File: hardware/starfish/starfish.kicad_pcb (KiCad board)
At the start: 4 copper layers, 80 x 70 mm, 164 parts, among them J1 INS, J10 Stemma QT, J2 8P8C_LED_Shielded, J3 CAM, J4 CAMLED, J5 OUT1, J6 BLTOUCH, J7 MOTOR, J8 MOTOR, J9 MOTOR, SW1 BOOTSEL, U1 VX7805-500, U10 TMC2209, U2 MIC5317-3.3, U3 RP2040, U4 W25Q128JVS, U5 74HC2G34, U6 TVS, U7 74HC2G34, U8 TMC2209, U9 TMC2209, Y1 12MHz

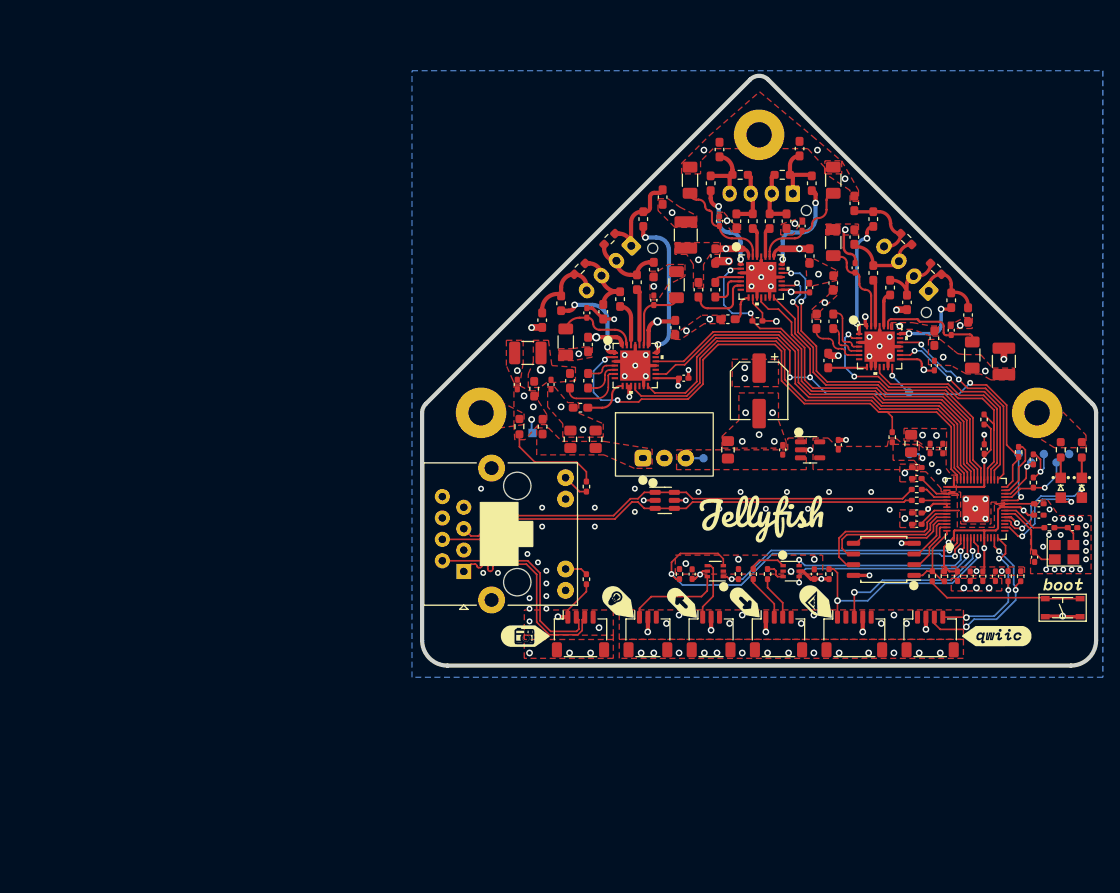
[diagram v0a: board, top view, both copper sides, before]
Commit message: First pass at layout and routing
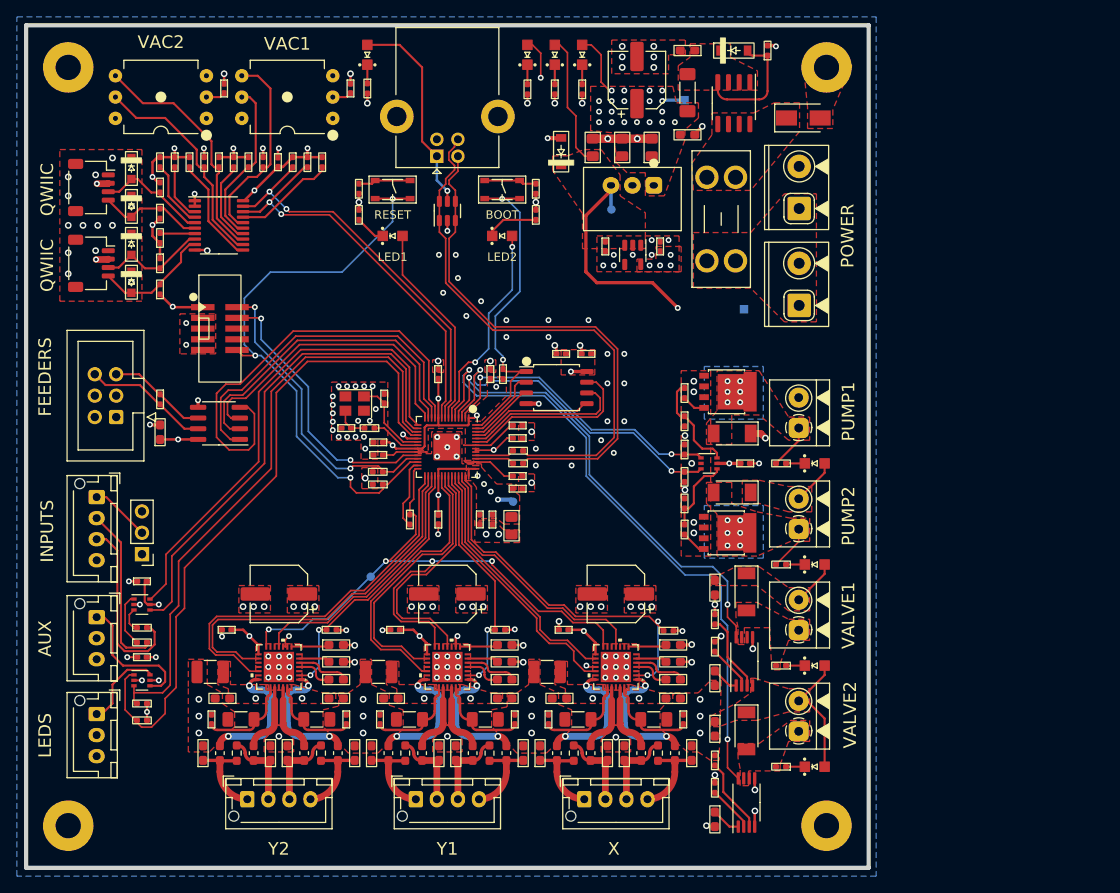
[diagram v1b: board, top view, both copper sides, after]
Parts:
- removed ? (x13): , Graphics
- removed C1, C27, C29, C32, C33, C43, C46, C47, C57, C60, C61, C8, C9: 100n, Capacitor_SMD:C_0402_1005Metric_Pad0.74x0.62mm_HandSolder
- removed C2: 4.7u, Capacitor_SMD:C_0805_2012Metric_Pad1.18x1.45mm_HandSolder
- removed C28, C42, C56: 22n, Capacitor_SMD:C_0603_1608Metric_Pad1.08x0.95mm_HandSolder
- removed C3, C4: 22u, Capacitor_SMD:C_0805_2012Metric_Pad1.18x1.45mm_HandSolder
- removed C30, C36, C37, C44, C50, C51, C58, C64, C65: 100n, Capacitor_SMD:C_0603_1608Metric_Pad1.08x0.95mm_HandSolder
- removed C31, C45, C59: 4.7u, Capacitor_SMD:C_0603_1608Metric_Pad1.08x0.95mm_HandSolder
- removed C35, C49, C63: 10u, Capacitor_SMD:C_1210_3225Metric_Pad1.33x2.70mm_HandSolder
- removed C38, C39, C40, C41, C52, C53, C54, C55, C66, C67, C68, C69: 470p, Capacitor_SMD:C_0603_1608Metric_Pad1.08x0.95mm_HandSolder
- removed C5: 100u, Capacitor_SMD:CP_Elec_6.3x7.7
- removed C6, C7: 1u, Capacitor_SMD:C_0402_1005Metric_Pad0.74x0.62mm_HandSolder
- removed FB1, FB10, FB11, FB12, FB13, FB14, FB2, FB3, FB4, FB5, FB6, FB7, FB8, FB9: 50Ω @ 100MHz, Inductor_SMD:L_0603_1608Metric_Pad1.05x0.95mm_HandSolder
- removed H1, H2, H3: GND, MountingHole:MountingHole_3mm_Pad
- removed J10: Stemma QT, Connector_JST:JST_SH_SM04B-SRSS-TB_1x04-1MP_P1.00mm_Horizontal
- removed J2: 8P8C_LED_Shielded, winterbloom:RJ45_Amphenol_RJE45-188-1411_Vertical
- removed J3: CAM, Connector_JST:JST_SH_SM04B-SRSS-TB_1x04-1MP_P1.00mm_Horizontal
- removed J4: CAMLED, Connector_JST:JST_SH_SM03B-SRSS-TB_1x03-1MP_P1.00mm_Horizontal
- removed J5: OUT1, Connector_JST:JST_SH_SM03B-SRSS-TB_1x03-1MP_P1.00mm_Horizontal
- removed J6: BLTOUCH, Connector_JST:JST_SH_SM05B-SRSS-TB_1x05-1MP_P1.00mm_Horizontal
- removed J7, J8, J9: MOTOR, Connector_JST:JST_XH_B4B-XH-AM_1x04_P2.50mm_Vertical
- removed R1, R15, R2, R26, R27: 5.1k, Resistor_SMD:R_0402_1005Metric_Pad0.72x0.64mm_HandSolder
- removed R13, R14, R20, R23: 10k, Resistor_SMD:R_0402_1005Metric_Pad0.72x0.64mm_HandSolder
- removed R16, R3: 100, Resistor_SMD:R_0402_1005Metric_Pad0.72x0.64mm_HandSolder
- removed R18, R19, R21, R22, R24, R25: 220m, Resistor_SMD:R_1206_3216Metric_Pad1.30x1.75mm_HandSolder
- removed RV1, RV2, RV3, RV4, RV5, RV6, RV7: 35V, Resistor_SMD:R_0603_1608Metric_Pad0.98x0.95mm_HandSolder
- removed TP1: GND, TestPoint:TestPoint_Pad_1.0x1.0mm
- removed TP2: 24V, TestPoint:TestPoint_Pad_1.0x1.0mm
- removed TP3: 5V, TestPoint:TestPoint_Pad_D1.0mm
- removed TP5: GND, TestPoint:TestPoint_Pad_D1.0mm
- removed TP6: 3V3, TestPoint:TestPoint_Pad_D1.0mm
- removed TP7: ~{RST}, TestPoint:TestPoint_Pad_D1.0mm
- removed TP8: SWD, TestPoint:TestPoint_Pad_D1.0mm
- removed TP9: SWC, TestPoint:TestPoint_Pad_D1.0mm
- removed U1: VX7805-500, winterbloom:Converter_DCDC_CUI_VX78-500_THT
- removed U10, U8, U9: TMC2209, winterbloom:TMC2209-LA
- removed U2: MIC5317-3.3, Package_TO_SOT_SMD:SOT-23-5
- removed U5, U7: 74HC2G34, Package_TO_SOT_SMD:SOT-363_SC-70-6
- removed U6: TVS, Package_TO_SOT_SMD:SOT-23-6
- added C1201: 4u7, winterbloom:C_0603_HandSolder, F.Cu at (100.0, 112.1)
- added C1202: 100n, winterbloom:C_0603_HandSolder, F.Cu at (100.0, 101.4)
- added C1301: 4u7, winterbloom:C_0603_HandSolder, F.Cu at (100.0, 128.9)
- added C1302: 100n, winterbloom:C_0603_HandSolder, F.Cu at (100.0, 118.1)
- added C1401: 22n, winterbloom:C_0603_HandSolder, F.Cu at (95.0, 112.3)
- added C1402: 100n, winterbloom:C_0402_HandSolder, F.Cu at (82.0, 106.4)
- added C1403: 100n, winterbloom:C_0603_HandSolder, F.Cu at (95.0, 110.2)
- added C1404: 4u7, winterbloom:C_0603_HandSolder, F.Cu at (95.0, 108.2)
- added C1405: 100n, winterbloom:C_0402_HandSolder, F.Cu at (96.2, 117.0)
- added C1406: 100n, winterbloom:C_0402_HandSolder, F.Cu at (80.2, 117.0)
- added C1407: 470p, winterbloom:C_0603_HandSolder, F.Cu at (89.2, 121.0)
- added C1408: 470p, winterbloom:C_0603_HandSolder, F.Cu at (79.2, 121.0)
- added C1409: 470p, winterbloom:C_0603_HandSolder, F.Cu at (97.2, 121.0)
- added C1410: 470p, winterbloom:C_0603_HandSolder, F.Cu at (87.2, 121.0)
- added C1411: 100u, Capacitor_SMD:CP_Elec_6.3x9.9, F.Cu at (68.2, 102.1)
- added C1412: 10u, winterbloom:C_1210_HandSolder, F.Cu at (80.0, 111.4)
- added C1413: 100n, winterbloom:C_0603_HandSolder, F.Cu at (95.0, 114.5)
- added C1414: 100n, winterbloom:C_0603_HandSolder, F.Cu at (81.5, 114.5)
- added C1501: 22n, winterbloom:C_0603_HandSolder, F.Cu at (75.0, 112.3)
- added C1502: 100n, winterbloom:C_0402_HandSolder, F.Cu at (62.0, 106.4)
- added C1503: 100n, winterbloom:C_0603_HandSolder, F.Cu at (75.0, 110.2)
- added C1504: 4u7, winterbloom:C_0603_HandSolder, F.Cu at (75.0, 108.2)
- added C1505: 100n, winterbloom:C_0402_HandSolder, F.Cu at (76.2, 117.0)
- added C1506: 100n, winterbloom:C_0402_HandSolder, F.Cu at (60.2, 117.0)
- added C1507: 470p, winterbloom:C_0603_HandSolder, F.Cu at (69.2, 121.0)
- added C1508: 470p, winterbloom:C_0603_HandSolder, F.Cu at (59.2, 121.0)
- added C1509: 470p, winterbloom:C_0603_HandSolder, F.Cu at (77.2, 121.0)
- added C1510: 470p, winterbloom:C_0603_HandSolder, F.Cu at (67.2, 121.0)
- added C1511: 100u, Capacitor_SMD:CP_Elec_6.3x9.9, F.Cu at (88.2, 102.1)
- added C1512: 10u, winterbloom:C_1210_HandSolder, F.Cu at (60.0, 111.4)
- added C1513: 100n, winterbloom:C_0603_HandSolder, F.Cu at (75.0, 114.5)
- added C1514: 100n, winterbloom:C_0603_HandSolder, F.Cu at (61.5, 114.5)
- added C1601: 22n, winterbloom:C_0603_HandSolder, F.Cu at (55.0, 112.3)
- added C1602: 100n, winterbloom:C_0402_HandSolder, F.Cu at (42.0, 106.4)
- added C1603: 100n, winterbloom:C_0603_HandSolder, F.Cu at (55.0, 110.2)
- added C1604: 4u7, winterbloom:C_0603_HandSolder, F.Cu at (55.0, 108.2)
- added C1605: 100n, winterbloom:C_0402_HandSolder, F.Cu at (56.2, 117.0)
- added C1606: 100n, winterbloom:C_0402_HandSolder, F.Cu at (40.2, 117.0)
- added C1607: 470p, winterbloom:C_0603_HandSolder, F.Cu at (49.2, 121.0)
- added C1608: 470p, winterbloom:C_0603_HandSolder, F.Cu at (39.2, 121.0)
- added C1609: 470p, winterbloom:C_0603_HandSolder, F.Cu at (57.2, 121.0)
- added C1610: 470p, winterbloom:C_0603_HandSolder, F.Cu at (47.2, 121.0)
- added C1611: 100u, Capacitor_SMD:CP_Elec_6.3x9.9, F.Cu at (48.2, 102.1)
- added C1612: 10u, winterbloom:C_1210_HandSolder, F.Cu at (40.0, 111.4)
- added C1613: 100n, winterbloom:C_0603_HandSolder, F.Cu at (55.0, 114.5)
- added C1614: 100n, winterbloom:C_0603_HandSolder, F.Cu at (41.5, 114.5)
- added C201: 100n, winterbloom:C_0603_HandSolder, F.Cu at (96.7, 37.6)
- added C202: 100n, winterbloom:C_0603_HandSolder, F.Cu at (96.7, 47.6)
- added C203: 100u, Capacitor_SMD:CP_Elec_6.3x9.9, F.Cu at (90.7, 41.1)
- added C206: 4u7, winterbloom:C_0805_HandSolder, F.Cu at (92.5, 49.1)
- added C207: 22u, winterbloom:C_0805_HandSolder, F.Cu at (89.0, 49.1)
- added C208: 22u, winterbloom:C_0805_HandSolder, F.Cu at (85.5, 49.1)
- added C209: 1u, winterbloom:C_0402_HandSolder, F.Cu at (87.0, 60.9)
- added C210: 1u, winterbloom:C_0402_HandSolder, F.Cu at (93.5, 60.9)
- added C401: 100n, winterbloom:C_0402_HandSolder, F.Cu at (31.9, 109.6)
- added C402: 100n, winterbloom:C_0402_HandSolder, F.Cu at (31.9, 100.6)
- added C501: 100n, winterbloom:C_0402_HandSolder, F.Cu at (48.1, 50.9)
- added C601: 100n, winterbloom:C_0402_HandSolder, F.Cu at (56.7, 42.1)
- added C701: 100n, winterbloom:C_0402_HandSolder, F.Cu at (41.7, 42.1)
- added C801: 100n, winterbloom:C_0603_HandSolder, F.Cu at (34.1, 82.9)
- added C901: 100n, winterbloom:C_0402_HandSolder, F.Cu at (103.6, 86.6)
- added D1001: On, winterbloom:LED_0805_Kingbright_APT2012, F.Cu at (111.8, 86.6)
- added D1002: PMEG3030EP, Diode_SMD:D_SOD-128, F.Cu at (102.0, 83.1)
- added D1101: On, winterbloom:LED_0805_Kingbright_APT2012, F.Cu at (111.8, 98.6)
- added D1102: PMEG3030EP, Diode_SMD:D_SOD-128, F.Cu at (102.0, 90.1)
- added D1201: On, winterbloom:LED_0805_Kingbright_APT2012, F.Cu at (111.8, 110.6)
- added D1202: PMEG3030EP, Diode_SMD:D_SOD-128, F.Cu at (103.7, 101.9)
- added D1301: On, winterbloom:LED_0805_Kingbright_APT2012, F.Cu at (111.8, 122.6)
- added D1302: PMEG3030EP, Diode_SMD:D_SOD-128, F.Cu at (103.7, 118.4)
- added D201: SMAJ28A, Diode_SMD:D_SMA, F.Cu at (110.5, 45.6)
- added D202: PDZ16BGWJ, winterbloom:D_SOD-123, F.Cu at (102.2, 37.6)
- added D203: 24V, winterbloom:LED_0805_Kingbright_APT2012, F.Cu at (84.2, 38.1)
- added D204: 5V, winterbloom:LED_0805_Kingbright_APT2012, F.Cu at (81.0, 38.1)
- added D205: 3V3, winterbloom:LED_0805_Kingbright_APT2012, F.Cu at (77.7, 38.1)
- added D401: PESD5V, winterbloom:D_SOD-323, F.Cu at (30.7, 51.6)
- added D402: PESD5V, winterbloom:D_SOD-323, F.Cu at (30.7, 60.6)
- added D403: PESD5V, winterbloom:D_SOD-323, F.Cu at (30.7, 56.1)
- added D404: PESD5V, winterbloom:D_SOD-323, F.Cu at (30.7, 65.1)
- added D405: PMEG2005EGWJ, winterbloom:D_SOD-123, F.Cu at (81.7, 49.6)
- added D406: USB, winterbloom:LED_0805_Kingbright_APT2012, F.Cu at (58.7, 38.1)
- added F201: Fuse, Fuse:Fuseholder_Blade_Mini_Keystone_3568, F.Cu at (99.0, 62.6)
- added FB1401: 120R @ 100MHz, Inductor_SMD:L_0603_1608Metric_Pad1.05x0.95mm_HandSolder, F.Cu at (95.2, 121.0)
- added FB1402: 120R @ 100MHz, Inductor_SMD:L_0603_1608Metric_Pad1.05x0.95mm_HandSolder, F.Cu at (91.2, 121.0)
- added FB1403: 120R @ 100MHz, Inductor_SMD:L_0603_1608Metric_Pad1.05x0.95mm_HandSolder, F.Cu at (85.2, 121.0)
- added FB1404: 120R @ 100MHz, Inductor_SMD:L_0603_1608Metric_Pad1.05x0.95mm_HandSolder, F.Cu at (81.2, 121.0)
- added FB1501: 120R @ 100MHz, Inductor_SMD:L_0603_1608Metric_Pad1.05x0.95mm_HandSolder, F.Cu at (75.2, 121.0)
- added FB1502: 120R @ 100MHz, Inductor_SMD:L_0603_1608Metric_Pad1.05x0.95mm_HandSolder, F.Cu at (71.2, 121.0)
- added FB1503: 120R @ 100MHz, Inductor_SMD:L_0603_1608Metric_Pad1.05x0.95mm_HandSolder, F.Cu at (65.2, 121.0)
- added FB1504: 120R @ 100MHz, Inductor_SMD:L_0603_1608Metric_Pad1.05x0.95mm_HandSolder, F.Cu at (61.2, 121.0)
- added FB1601: 120R @ 100MHz, Inductor_SMD:L_0603_1608Metric_Pad1.05x0.95mm_HandSolder, F.Cu at (55.2, 121.0)
- added FB1602: 120R @ 100MHz, Inductor_SMD:L_0603_1608Metric_Pad1.05x0.95mm_HandSolder, F.Cu at (51.2, 121.0)
- added FB1603: 120R @ 100MHz, Inductor_SMD:L_0603_1608Metric_Pad1.05x0.95mm_HandSolder, F.Cu at (45.2, 121.0)
- added FB1604: 120R @ 100MHz, Inductor_SMD:L_0603_1608Metric_Pad1.05x0.95mm_HandSolder, F.Cu at (41.2, 121.0)
- added FB201: 60R @ 100MHz, Inductor_SMD:L_1806_4516Metric_Pad1.45x1.90mm_HandSolder, F.Cu at (96.7, 42.6)
- added H101: GND, MountingHole:MountingHole_3mm_Pad, F.Cu at (23.2, 39.6)
- added H102: GND, MountingHole:MountingHole_3mm_Pad, F.Cu at (113.2, 39.6)
- added H103: GND, MountingHole:MountingHole_3mm_Pad, F.Cu at (23.2, 129.6)
- added H104: GND, MountingHole:MountingHole_3mm_Pad, F.Cu at (113.2, 129.6)
- added J1001: Pump, winterbloom:TerminalBlock_4UCON_1x02_P3.50mm_Horizontal, F.Cu at (109.9, 82.4)
- added J1101: Pump, winterbloom:TerminalBlock_4UCON_1x02_P3.50mm_Horizontal, F.Cu at (109.9, 94.4)
- added J1201: Valve, winterbloom:TerminalBlock_4UCON_1x02_P3.50mm_Horizontal, F.Cu at (109.9, 106.4)
- added J1301: Valve, winterbloom:TerminalBlock_4UCON_1x02_P3.50mm_Horizontal, F.Cu at (109.9, 118.4)
- added J1401: Motor, Connector_JST:JST_XH_B4B-XH-AM_1x04_P2.50mm_Vertical, F.Cu at (84.5, 126.5)
- added J1501: Motor, Connector_JST:JST_XH_B4B-XH-AM_1x04_P2.50mm_Vertical, F.Cu at (64.5, 126.5)
- added J1601: Motor, Connector_JST:JST_XH_B4B-XH-AM_1x04_P2.50mm_Vertical, F.Cu at (44.5, 126.5)
- added J201: DC in, winterbloom:TerminalBlock_CUI_TB002-500_1x02_P5.00mm_Vertical, F.Cu at (110.0, 56.4)
- added J202: DC thru, winterbloom:TerminalBlock_CUI_TB002-500_1x02_P5.00mm_Vertical, F.Cu at (110.0, 67.9)
- added J401: Cam LED, Connector_JST:JST_XH_B3B-XH-AM_1x03_P2.50mm_Vertical, F.Cu at (26.6, 116.4)
- added J402: Aux out, Connector_JST:JST_XH_B3B-XH-AM_1x03_P2.50mm_Vertical, F.Cu at (26.6, 104.9)
- added J403: Voltage, Connector_PinHeader_2.54mm:PinHeader_1x03_P2.54mm_Vertical, F.Cu at (31.9, 97.4)
- added J404: Inputs, Connector_JST:JST_XH_B4B-XH-AM_1x04_P2.50mm_Vertical, F.Cu at (26.6, 90.6)
- added J405: Qwiic, Connector_JST:JST_SH_SM04B-SRSS-TB_1x04-1MP_P1.00mm_Horizontal, F.Cu at (25.9, 53.9)
- added J406: Qwiic, Connector_JST:JST_SH_SM04B-SRSS-TB_1x04-1MP_P1.00mm_Horizontal, F.Cu at (25.9, 62.9)
- added J407: USB B, winterbloom:USB_B_Receptacle_Horizontal, F.Cu at (67.0, 50.1)
- added J801: Feeders, Connector_IDC:IDC-Header_2x03_P2.54mm_Vertical, F.Cu at (28.9, 81.1)
- added Q1001: PSMN011-30YLC, Package_TO_SOT_SMD:LFPAK56, F.Cu at (101.5, 78.1)
- added Q1101: PSMN011-30YLC, Package_TO_SOT_SMD:LFPAK56, F.Cu at (101.5, 94.9)
- added Q201: DMP3037LSS-13, Package_SO:SOIC-8_3.9x4.9mm_P1.27mm, F.Cu at (102.2, 43.9)
- added R1001: 100k, winterbloom:R_0402_HandSolder, F.Cu at (96.3, 81.6)
- added R1002: 1k, winterbloom:R_0402_HandSolder, F.Cu at (96.3, 78.3)
- added R1003: 5k1, winterbloom:R_0402_HandSolder, F.Cu at (107.8, 86.6)
- added R1101: 100k, winterbloom:R_0402_HandSolder, F.Cu at (96.3, 91.4)
- added R1102: 1k, winterbloom:R_0402_HandSolder, F.Cu at (96.3, 94.5)
- added R1103: 5k1, winterbloom:R_0402_HandSolder, F.Cu at (107.8, 98.6)
- added R1201: 0R, winterbloom:R_0402_HandSolder, F.Cu at (100.0, 105.1)
- added R1202: 47k, winterbloom:R_0402_HandSolder, F.Cu at (100.0, 108.4)
- added R1203: 5k1, winterbloom:R_0402_HandSolder, F.Cu at (107.8, 110.6)
- added R1301: 0R, winterbloom:R_0402_HandSolder, F.Cu at (100.0, 121.9)
- added R1302: 47k, winterbloom:R_0402_HandSolder, F.Cu at (100.0, 125.1)
- added R1303: 5k1, winterbloom:R_0402_HandSolder, F.Cu at (107.8, 122.6)
- added R1402: 120m, Resistor_SMD:R_1206_3216Metric_Pad1.30x1.75mm_HandSolder, F.Cu at (92.7, 117.0)
- added R1403: 120m, Resistor_SMD:R_1206_3216Metric_Pad1.30x1.75mm_HandSolder, F.Cu at (83.7, 117.0)
- added R1501: 10k, winterbloom:R_0402_HandSolder, F.Cu at (74.5, 106.4)
- added R1502: 120m, Resistor_SMD:R_1206_3216Metric_Pad1.30x1.75mm_HandSolder, F.Cu at (72.7, 117.0)
- added R1503: 120m, Resistor_SMD:R_1206_3216Metric_Pad1.30x1.75mm_HandSolder, F.Cu at (63.7, 117.0)
- added R1601: 10k, winterbloom:R_0402_HandSolder, F.Cu at (54.5, 106.4)
- added R1602: 120m, Resistor_SMD:R_1206_3216Metric_Pad1.30x1.75mm_HandSolder, F.Cu at (52.7, 117.0)
- added R1603: 120m, Resistor_SMD:R_1206_3216Metric_Pad1.30x1.75mm_HandSolder, F.Cu at (43.7, 117.0)
- added R201: 47k, winterbloom:R_0402_HandSolder, F.Cu at (106.2, 37.6)
- added R202: 5k1, winterbloom:R_0402_HandSolder, F.Cu at (84.2, 42.2)
- added R203: 1k, winterbloom:R_0402_HandSolder, F.Cu at (81.0, 42.2)
- added R204: 1k, winterbloom:R_0402_HandSolder, F.Cu at (77.7, 42.2)
- added R306: 1k, winterbloom:R_0402_HandSolder, F.Cu at (57.7, 54.0)
- added R401: 10k, winterbloom:R_0402_HandSolder, F.Cu at (31.9, 117.1)
- added R402: 10k, winterbloom:R_0402_HandSolder, F.Cu at (31.9, 115.1)
- added R403: 120R, winterbloom:R_0402_HandSolder, F.Cu at (31.9, 107.9)
- added R404: 120R, winterbloom:R_0402_HandSolder, F.Cu at (31.9, 106.1)
- added R405: 1k, winterbloom:R_0402_HandSolder, F.Cu at (58.7, 42.1)
- added R501: 4k7, winterbloom:R_0402_HandSolder, F.Cu at (51.6, 50.9)
- added R502: 4k7, winterbloom:R_0402_HandSolder, F.Cu at (49.8, 50.9)
- added R503: 10k, winterbloom:R_0402_HandSolder, F.Cu at (53.3, 50.9)
- added R504: 10k, winterbloom:R_0402_HandSolder, F.Cu at (35.8, 50.9)
- added R505: 10k, winterbloom:R_0402_HandSolder, F.Cu at (34.1, 50.9)
- added R506: 4k7, winterbloom:R_0402_HandSolder, F.Cu at (34.1, 53.9)
- added R507: 4k7, winterbloom:R_0402_HandSolder, F.Cu at (34.1, 57.0)
- added R508: 10k, winterbloom:R_0402_HandSolder, F.Cu at (34.1, 59.9)
- added R509: 4k7, winterbloom:R_0402_HandSolder, F.Cu at (34.1, 62.9)
- added R510: 4k7, winterbloom:R_0402_HandSolder, F.Cu at (34.1, 66.0)
- added R511: 10k, winterbloom:R_0402_HandSolder, F.Cu at (37.6, 50.9)
- added R512: 4k7, winterbloom:R_0402_HandSolder, F.Cu at (39.3, 50.9)
- added R513: 4k7, winterbloom:R_0402_HandSolder, F.Cu at (41.1, 50.9)
- added R514: 10k, winterbloom:R_0402_HandSolder, F.Cu at (42.8, 50.9)
- added R515: 4k7, winterbloom:R_0402_HandSolder, F.Cu at (44.6, 50.9)
- added R516: 4k7, winterbloom:R_0402_HandSolder, F.Cu at (46.3, 50.9)
- added R801: 120R, winterbloom:R_0402_HandSolder, F.Cu at (34.1, 79.0)
- added R901: 10k, winterbloom:R_0402_HandSolder, F.Cu at (96.3, 85.0)
- added R902: 10k, winterbloom:R_0402_HandSolder, F.Cu at (96.3, 88.2)
- added RV1401: MOV, Resistor_SMD:R_0603_1608Metric_Pad0.98x0.95mm_HandSolder, F.Cu at (93.2, 121.0)
- added RV1402: MOV, Resistor_SMD:R_0603_1608Metric_Pad0.98x0.95mm_HandSolder, F.Cu at (83.2, 121.0)
- added RV1501: MOV, Resistor_SMD:R_0603_1608Metric_Pad0.98x0.95mm_HandSolder, F.Cu at (73.2, 121.0)
- added RV1502: MOV, Resistor_SMD:R_0603_1608Metric_Pad0.98x0.95mm_HandSolder, F.Cu at (63.2, 121.0)
- added RV1601: MOV, Resistor_SMD:R_0603_1608Metric_Pad0.98x0.95mm_HandSolder, F.Cu at (53.2, 121.0)
- added RV1602: MOV, Resistor_SMD:R_0603_1608Metric_Pad0.98x0.95mm_HandSolder, F.Cu at (43.2, 121.0)
- added SW301: RESET, winterbloom:Tactile_Switch_4.2mm, F.Cu at (61.7, 54.1)
- added TP201: GND, TestPoint:TestPoint_Pad_1.0x1.0mm, B.Cu at (103.4, 68.3)
- added TP202: 24V, TestPoint:TestPoint_Pad_1.0x1.0mm, B.Cu at (96.3, 43.5)
- added TP203: 5V, TestPoint:TestPoint_Pad_D1.0mm, B.Cu at (87.7, 56.5)
- added U1201: DRV120PWR, Package_SO:TSSOP-8_4.4x3mm_P0.65mm, F.Cu at (103.5, 110.1)
- added U1301: DRV120PWR, Package_SO:TSSOP-8_4.4x3mm_P0.65mm, F.Cu at (103.7, 126.9)
- added U1401: TMC2209, winterbloom:TMC2209-LA, F.Cu at (88.2, 110.8)
- added U1501: TMC2209, winterbloom:TMC2209-LA, F.Cu at (68.2, 110.8)
- added U1601: TMC2209, winterbloom:TMC2209-LA, F.Cu at (48.2, 110.8)
- added U201: VX7805-500, winterbloom:Converter_DCDC_CUI_VX78-500_THT, F.Cu at (92.7, 53.6)
- added U202: MIC5317-3.3, Package_TO_SOT_SMD:SOT-23-5, F.Cu at (90.2, 61.9)
- added U401: 74HC2G34, Package_TO_SOT_SMD:SOT-363_SC-70-6, F.Cu at (31.9, 112.4)
- added U402: 74HC2G34, Package_TO_SOT_SMD:SOT-363_SC-70-6, F.Cu at (31.9, 103.4)
- added U403: TVS, Package_TO_SOT_SMD:SOT-23-6, F.Cu at (68.2, 56.6)
- added U501: PCA9545, Package_SO:TSSOP-20_4.4x6.5mm_P0.65mm, F.Cu at (41.1, 58.4)
- added U601: XGZP6857D, winterbloom:XGZP6857D, F.Cu at (49.2, 43.1)
- added U701: XGZP6857D, winterbloom:XGZP6857D, F.Cu at (34.2, 43.1)
- added U801: MAX3078E, Package_SO:SOIC-8_3.9x4.9mm_P1.27mm, F.Cu at (41.1, 81.9)
- added U901: 74HC2G34, Package_TO_SOT_SMD:SOT-363_SC-70-6, F.Cu at (99.2, 86.6)
- C301: renamed from C10; footprint Capacitor_SMD:C_0805_2012Metric_Pad1.18x1.45mm_HandSolder -> winterbloom:C_0805_HandSolder
- C302: renamed from C11; footprint Capacitor_SMD:C_0402_1005Metric_Pad0.74x0.62mm_HandSolder -> winterbloom:C_0402_HandSolder
- C303: renamed from C12; footprint Capacitor_SMD:C_0402_1005Metric_Pad0.74x0.62mm_HandSolder -> winterbloom:C_0402_HandSolder
- C304: renamed from C13; footprint Capacitor_SMD:C_0402_1005Metric_Pad0.74x0.62mm_HandSolder -> winterbloom:C_0402_HandSolder
- C305: renamed from C14; footprint Capacitor_SMD:C_0402_1005Metric_Pad0.74x0.62mm_HandSolder -> winterbloom:C_0402_HandSolder
- C306: renamed from C15; footprint Capacitor_SMD:C_0402_1005Metric_Pad0.74x0.62mm_HandSolder -> winterbloom:C_0402_HandSolder
- C307: renamed from C16; footprint Capacitor_SMD:C_0402_1005Metric_Pad0.74x0.62mm_HandSolder -> winterbloom:C_0402_HandSolder
- C308: renamed from C17; footprint Capacitor_SMD:C_0402_1005Metric_Pad0.74x0.62mm_HandSolder -> winterbloom:C_0402_HandSolder
- C309: renamed from C18; footprint Capacitor_SMD:C_0402_1005Metric_Pad0.74x0.62mm_HandSolder -> winterbloom:C_0402_HandSolder
- C310: renamed from C19; footprint Capacitor_SMD:C_0402_1005Metric_Pad0.74x0.62mm_HandSolder -> winterbloom:C_0402_HandSolder
- C311: renamed from C20; footprint Capacitor_SMD:C_0402_1005Metric_Pad0.74x0.62mm_HandSolder -> winterbloom:C_0402_HandSolder
- C312: renamed from C21; footprint Capacitor_SMD:C_0402_1005Metric_Pad0.74x0.62mm_HandSolder -> winterbloom:C_0402_HandSolder
- C313: renamed from C23; footprint Capacitor_SMD:C_0402_1005Metric_Pad0.74x0.62mm_HandSolder -> winterbloom:C_0402_HandSolder
- C314: renamed from C24; footprint Capacitor_SMD:C_0402_1005Metric_Pad0.74x0.62mm_HandSolder -> winterbloom:C_0402_HandSolder
- C315: renamed from C25; footprint Capacitor_SMD:C_0402_1005Metric_Pad0.74x0.62mm_HandSolder -> winterbloom:C_0402_HandSolder
- C316: renamed from C26; footprint Capacitor_SMD:C_0402_1005Metric_Pad0.74x0.62mm_HandSolder -> winterbloom:C_0402_HandSolder
- D301: renamed from D4; value ACT -> Act
- D302: renamed from D1; value AUX -> Aux
- J1: value INS -> SWD; footprint Connector_JST:JST_SH_SM04B-SRSS-TB_1x04-1MP_P1.00mm_Horizontal -> winterbloom:Connector_Cortex_Debug_IDC_2x05_P1.27mm_Vertical_Shrouded_SMD
- R1401: renamed from R17; footprint Resistor_SMD:R_0402_1005Metric_Pad0.72x0.64mm_HandSolder -> winterbloom:R_0402_HandSolder
- R301: renamed from R4; footprint Resistor_SMD:R_0402_1005Metric_Pad0.72x0.64mm_HandSolder -> winterbloom:R_0402_HandSolder
- R302: renamed from R5; footprint Resistor_SMD:R_0402_1005Metric_Pad0.72x0.64mm_HandSolder -> winterbloom:R_0402_HandSolder
- R303: renamed from R6; footprint Resistor_SMD:R_0402_1005Metric_Pad0.72x0.64mm_HandSolder -> winterbloom:R_0402_HandSolder
- R304: renamed from R7; footprint Resistor_SMD:R_0402_1005Metric_Pad0.72x0.64mm_HandSolder -> winterbloom:R_0402_HandSolder
- R305: renamed from R8; footprint Resistor_SMD:R_0402_1005Metric_Pad0.72x0.64mm_HandSolder -> winterbloom:R_0402_HandSolder
- R307: renamed from R9; footprint Resistor_SMD:R_0402_1005Metric_Pad0.72x0.64mm_HandSolder -> winterbloom:R_0402_HandSolder
- R308: renamed from R10; footprint Resistor_SMD:R_0603_1608Metric_Pad0.98x0.95mm_HandSolder -> winterbloom:R_0402_HandSolder
- R309: renamed from R28; footprint Resistor_SMD:R_0603_1608Metric_Pad0.98x0.95mm_HandSolder -> winterbloom:R_0402_HandSolder
- R310: renamed from R11; footprint Resistor_SMD:R_0402_1005Metric_Pad0.72x0.64mm_HandSolder -> winterbloom:R_0402_HandSolder
- R311: renamed from R12; footprint Resistor_SMD:R_0402_1005Metric_Pad0.72x0.64mm_HandSolder -> winterbloom:R_0402_HandSolder
- moved R308 90.2 mm to (57.7, 57.1)
- moved D301 87.1 mm to (61.7, 59.6), turned to 0 degrees
- moved C314 87.0 mm to (56.2, 82.4), turned to 180 degrees
- moved Y301 86.0 mm to (57.2, 79.5), turned to 180 degrees
- moved SW302 83.0 mm to (74.7, 54.1), turned to 180 degrees
- moved R310 81.6 mm to (59.0, 82.4), turned to 180 degrees
- moved C313 79.5 mm to (60.7, 78.9), turned to 90 degrees
- moved C303 78.9 mm to (60.0, 84.1), turned to 180 degrees
- moved C312 78.6 mm to (60.0, 85.6), turned to 180 degrees
- moved R301 77.9 mm to (60.0, 89.1), turned to 180 degrees
- moved R302 77.8 mm to (59.9, 87.6), turned to 0 degrees
- moved J1 75.6 mm to (41.2, 70.6)
- moved D302 72.7 mm to (74.7, 59.6), turned to 0 degrees
- moved R305 72.7 mm to (63.8, 93.3)
- moved C302 69.0 mm to (67.1, 76.0), turned to 90 degrees
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- renumbered SW1 to SW302, TP4 to TP204, TP17 to TP301, U3 to U301, U4 to U302, Y1 to Y301
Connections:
- J1 pad 1: +5V -> +3V3
- J1 pad 2: Net-(R3-Pad2) -> /Microcontroller/SWD
- J1 pad 3: Net-(R16-Pad2) -> GND
- J1 pad 4: GND -> /Microcontroller/SWCLK
- R1401 pad 1: /Left Motor/ENN -> /Microcontroller/M0_EN
- R303 pad 1: /Microcontroller/USB_D+ -> /Connections/MCU_D+
- R304 pad 1: /Microcontroller/USB_D- -> /Connections/MCU_D-
- R305 pad 1: /Microcontroller/UART1_TX -> /TMC_UART
- R305 pad 2: /TMC_UART -> /Microcontroller/UART0_TX
- R307 pad 1: Net-(R9-Pad1) -> GND
- R307 pad 2: /Microcontroller/QSPI_CS -> Net-(R307-Pad2)
- SW302 pad 1: Net-(R9-Pad1) -> /Microcontroller/QSPI_CS
- SW302 pad 2: GND -> Net-(R307-Pad2)
- U301 pad 11: unconnected-(U3-Pad11) -> /Microcontroller/UART1_TX
- U301 pad 12: unconnected-(U3-Pad12) -> /Microcontroller/UART1_RX
- U301 pad 13: /Connections/QWIIC_SDA -> /Microcontroller/RS485_~{IN_EN}
- U301 pad 14: /Connections/QWIIC_SCL -> /Microcontroller/RS485_OUT_EN
- U301 pad 15: unconnected-(U3-Pad15) -> /Connections/IN_1
- U301 pad 16: /Microcontroller/AUX_LED -> /Connections/IN_2
- U301 pad 17: unconnected-(U3-Pad17) -> /Connections/AUX_OUT
- U301 pad 18: /Microcontroller/ACT_LED -> /Connections/CAM_LED
- U301 pad 2: /Connections/CAM_LED -> /Buffer/IN_A
- U301 pad 27: /Microcontroller/UART1_TX -> /Microcontroller/UART0_TX
- U301 pad 29: /Left Motor/DIR -> /Microcontroller/M2_DIR
- U301 pad 3: /Connections/AUX_OUT -> /Buffer/IN_B
- U301 pad 30: /Left Motor/STEP -> /Microcontroller/M2_STEP
- U301 pad 31: /Left Motor/DIAG -> /Microcontroller/M2_DIAG
- U301 pad 32: /Left Motor/ENN -> /Microcontroller/M2_EN
- U301 pad 38: /Microcontroller/M2_DIR -> /Microcontroller/M0_DIR
- U301 pad 39: /Microcontroller/M2_STEP -> /Microcontroller/M0_STEP
- U301 pad 4: /Connections/IN_1 -> /Microcontroller/VALVE_A
- U301 pad 40: /Microcontroller/M2_DIAG -> /Microcontroller/M0_DIAG
- U301 pad 41: /Microcontroller/M2_EN -> /Microcontroller/M0_EN
- U301 pad 5: /Connections/IN_2 -> /Microcontroller/VALVE_B
- U301 pad 6: /Connections/BLTOUCH_CONTROL -> /Microcontroller/AUX_LED
- U301 pad 7: /Connections/BLTOUCH_OUT -> /Microcontroller/ACT_LED
- U301 pad 8: unconnected-(U3-Pad8) -> /Microcontroller/I2C1_SDA
- U301 pad 9: unconnected-(U3-Pad9) -> /Microcontroller/I2C1_SCL
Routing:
- net +3V3: track 162.3 -> 479.1 mm, vias 20 -> 38
- net +24V: track 13.3 -> 295.5 mm, vias 3 -> 39
- net +5V: track 80.5 -> 215.7 mm, vias 7 -> 4
- net /Microcontroller/VALVE_B: track 0.00 -> 75.2 mm, vias 0 -> 2
- net /Connections/MCU_D+: track 0.00 -> 63.8 mm
- net /Microcontroller/RUN: track 6.29 -> 69.7 mm, vias 1 -> 3
- net /Connections/MCU_D-: track 0.00 -> 62.3 mm
- net /Microcontroller/USB_D+: track 58.2 -> 0.00 mm
- net /Microcontroller/USB_D-: track 56.4 -> 0.00 mm
- net /Microcontroller/VALVE_A: track 0.00 -> 56.0 mm, vias 0 -> 2
- net /Connections/CAM_LED: track 31.1 -> 80.1 mm, vias 2 -> 0
- net Net-(D405-Pad2): track 0.00 -> 48.0 mm, vias 0 -> 2
- net /Microcontroller/I2C1_SCL: track 0.00 -> 47.6 mm, vias 0 -> 2
- net /Microcontroller/I2C1_SDA: track 0.00 -> 46.8 mm, vias 0 -> 2
- net /Microcontroller/UART1_TX: track 7.05 -> 53.1 mm
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- added copper zone on F.Cu, net /Power/DCIN
- added copper zone on F.Cu, net /Power/post fuse
- added copper zone on F.Cu, net /Power/post polarity
- added copper zone on B.Cu, net /Pump A/switched
- added copper zone on F.Cu, net /Pump A/switched
- added copper zone on B.Cu, net /Pump B/switched
- added copper zone on F.Cu, net /Pump B/switched
- added copper zone on F.Cu, net /Valve A/switched
- added copper zone on F.Cu, net /Valve B/switched
- removed copper zone on F.Cu, net /Power/VIN_FILTERED
- removed copper zone on F.Cu, net VMOTOR
- removed copper zone on In2.Cu, net VMOTOR
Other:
- board size 80 x 70 mm -> 100 x 100 mm
- board text added: "AUX"
- board text added: "BOOT"
- board text added: "FEEDERS"
- board text added: "INPUTS"
- board text added: "LED1"
- board text added: "LED2"
- board text added: "LEDS"
- board text added: "POWER"
- board text added: "PUMP1"
- board text added: "PUMP2"
- board text added: "QWIIC"
- board text added: "RESET"
- board text added: "TODO: Heatsinking"
- board text added: "VAC1"
- board text added: "VAC2"
- board text added: "VALVE1"
- board text added: "VALVE2"
- board text added: "X"
- board text added: "Y1"
- board text added: "Y2"
- board text removed: "${COMMENT1} ${COMMENT2}"
- board text removed: "${COMPANY} ${COMMENT3} ${REVISION} ${ISSUE_DATE}"
